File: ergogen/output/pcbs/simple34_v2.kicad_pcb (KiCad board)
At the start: 2 copper layers, 122.2 x 90.8 mm, 42 parts

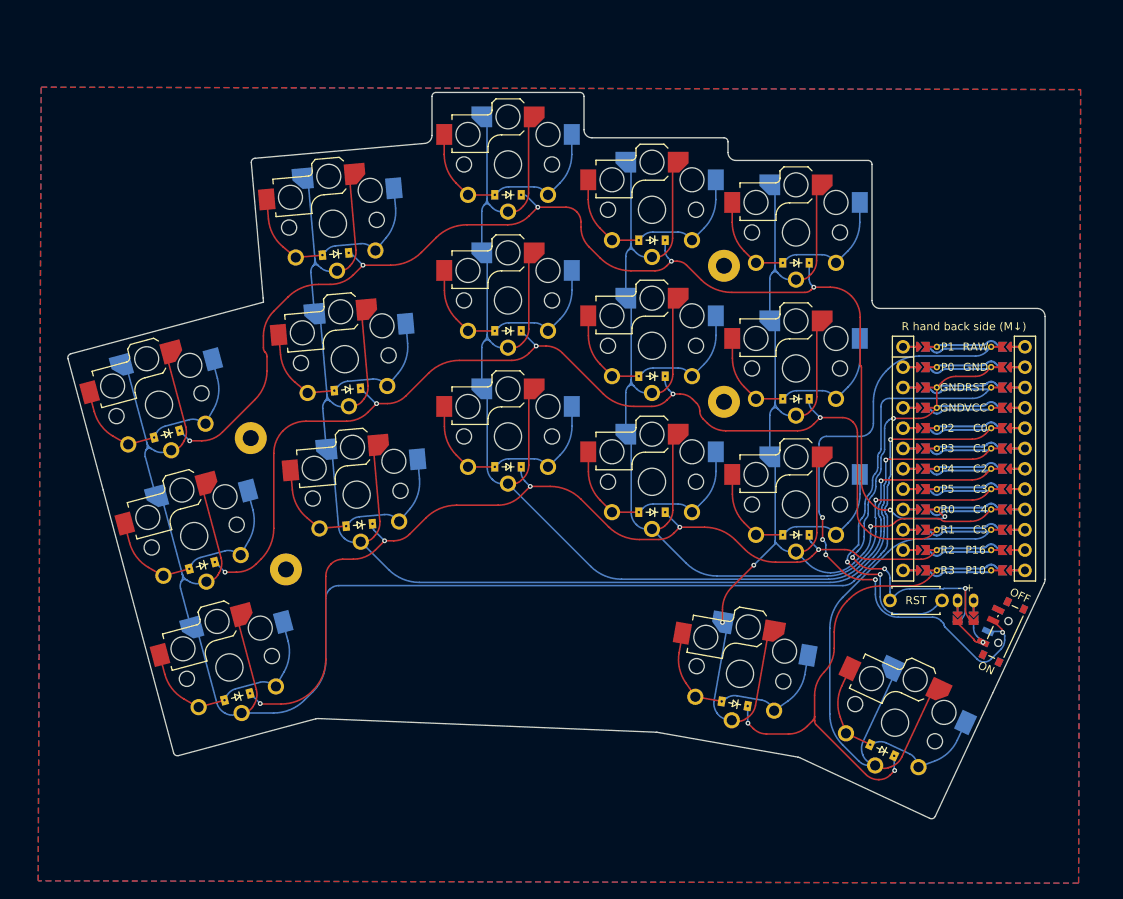
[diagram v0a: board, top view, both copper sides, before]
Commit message: OH MY, ARCS EXISTS
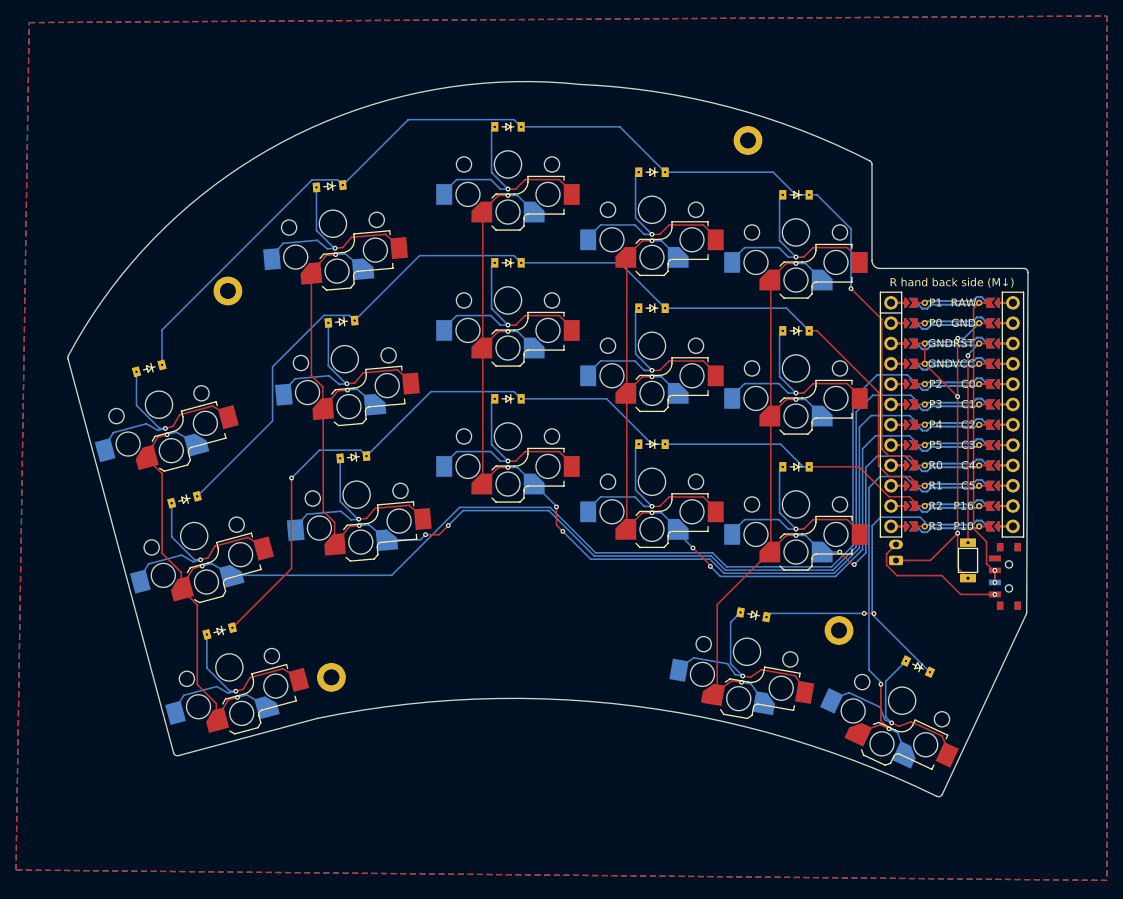
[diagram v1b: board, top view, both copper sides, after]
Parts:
- removed RST1: , ceoloide:reset_switch_tht_top
- added SW1: , local:reset_smd, F.Cu at (137.9, 87.2)
- moved H4 32.0 mm to (121.8, 96.0), turned to -17.5 degrees
- moved H1 18.6 mm to (45.4, 53.5)
- moved H2 16.0 mm to (110.4, 34.7)
- moved H3 14.6 mm to (58.4, 101.8)
- moved D17 11.4 mm to (131.7, 100.5)
- moved D16 11.4 mm to (111.1, 94.0)
- moved JST1 10.6 mm to (128.9, 86.2), turned to 90 degrees
- moved D6 8.50 mm to (58.1, 40.4)
- moved D4 8.50 mm to (61.1, 74.3)
- moved D5 8.50 mm to (59.6, 57.4)
- moved D14 8.50 mm to (116.4, 58.5)
- moved D10 8.50 mm to (98.4, 72.7)
- moved D12 8.50 mm to (98.4, 38.7)
- moved D13 8.50 mm to (116.4, 75.5)
- moved D15 8.50 mm to (116.4, 41.5)
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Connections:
- JST1 pad 1: BAT_P -> GND
- JST1 pad 2: GND -> BAT_P
- S1 pad 1: pinky_bottom -> C0
- S10 pad 1: index_bottom -> C3
- S11 pad 1: index_home -> C3
- S12 pad 1: index_top -> C3
- S13 pad 1: inner_bottom -> C4
- S14 pad 1: inner_home -> C4
- S15 pad 1: inner_top -> C4
- S16 pad 1: first_only -> C4
- S17 pad 1: second_only -> C5
- S2 pad 1: pinky_home -> C0
- S3 pad 1: pinky_top -> C0
- S4 pad 1: ring_bottom -> C1
- S5 pad 1: ring_home -> C1
- S6 pad 1: ring_top -> C1
- S7 pad 1: middle_bottom -> C2
- S8 pad 1: middle_home -> C2
- S9 pad 1: middle_top -> C2
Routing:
- net C4: track 177.6 -> 122.3 mm, vias 3 -> 6
- net C0: track 229.2 -> 184.3 mm, vias 1 -> 3
- net C3: track 159.5 -> 116.6 mm, vias 1 -> 5
- net C2: track 182.7 -> 140.1 mm, vias 1 -> 5
- net C1: track 200.9 -> 160.0 mm, vias 1 -> 5
- net RAW: track 88.5 -> 47.8 mm, vias 5 -> 2
- net C5: track 83.2 -> 56.0 mm, vias 0 -> 2
- net RST: track 62.1 -> 35.3 mm, vias 2 -> 1
- net R1: track 148.4 -> 134.1 mm, vias 5 -> 0
- net R0: track 165.5 -> 151.7 mm, vias 7 -> 1
- net R3: track 65.5 -> 52.6 mm
- net BAT_P: track 7.03 -> 18.1 mm
- net GND: track 91.0 -> 81.0 mm, vias 4 -> 3
- net R2: track 129.5 -> 120.8 mm, vias 5 -> 1
- net JST1_2: track 3.60 -> 0.00 mm
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- added copper zone on B.Cu, net GND
- added copper zone on F.Cu, net GND
- removed copper zone on B.Cu, net (none)
- removed copper zone on F.Cu, net (none)
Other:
- board size 122.2 x 90.8 mm -> 120 x 89.4 mm
- board text removed: "- +"

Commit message: case fillet
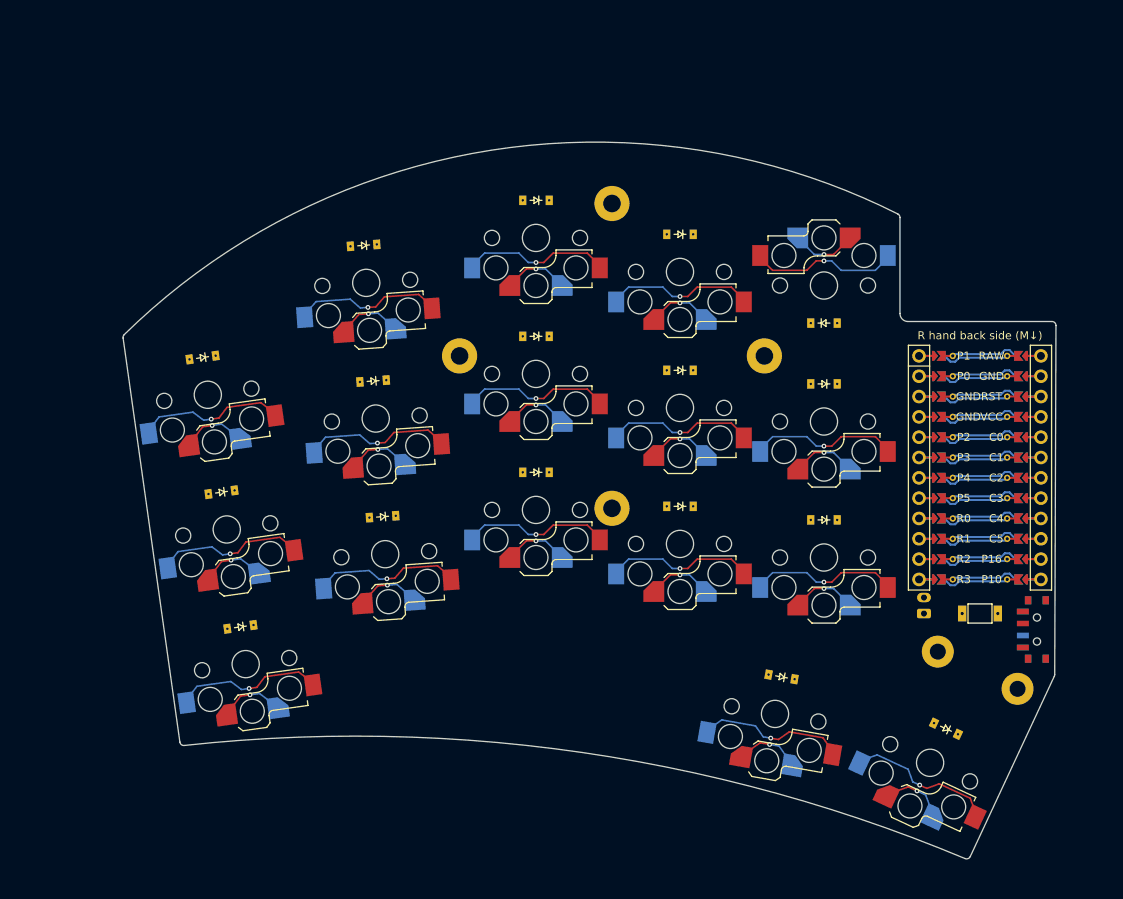
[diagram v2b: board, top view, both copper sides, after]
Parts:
- removed H3, H4: , ceoloide:mounting_hole_plated
- added TP1: Tenting Puck, no hole, TentingPuck_NoHole, B.Cu at (93.4, 61.6)
- moved H1 99.5 mm to (134.2, 98.6), turned to -25 degrees
- moved H2 76.4 mm to (144.1, 103.3), turned to -25 degrees
- moved D15 16.4 mm to (119.9, 57.5), turned to 360 degrees
- moved S7 9.83 mm to (83.9, 80.9)
- moved D8 9.83 mm to (83.9, 59.2)
- moved D9 9.83 mm to (83.9, 42.2)
- moved S8 9.83 mm to (83.9, 63.9)
- moved S9 9.83 mm to (83.9, 46.9)
- moved D7 9.83 mm to (83.9, 76.2)
- moved D6 8.52 mm to (62.4, 47.8), turned to 184 degrees
- moved D10 8.52 mm to (101.9, 80.4)
- moved S11 8.52 mm to (101.9, 68.1)
- moved S12 8.52 mm to (101.9, 51.1)
- moved D11 8.52 mm to (101.9, 63.4)
- moved D12 8.52 mm to (101.9, 46.4)
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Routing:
- net (no net): track 0.00 -> 337.7 mm
- net C0: track 184.3 -> 24.8 mm
- net R0: track 151.7 -> 0.00 mm, vias 1 -> 0
- net C1: track 160.0 -> 24.8 mm, vias 5 -> 3
- net R1: track 134.1 -> 0.00 mm
- net R2: track 120.8 -> 0.00 mm, vias 1 -> 0
- net C2: track 140.1 -> 24.8 mm, vias 5 -> 3
- net C3: track 116.6 -> 24.8 mm, vias 5 -> 3
- net C4: track 122.3 -> 33.1 mm, vias 6 -> 4
- net GND: track 81.0 -> 0.00 mm, vias 3 -> 0
- net R3: track 52.6 -> 0.00 mm, vias 2 -> 0
- net RAW: track 47.8 -> 0.00 mm, vias 2 -> 0
- net C5: track 56.0 -> 8.27 mm, vias 2 -> 1
- net RST: track 35.3 -> 0.00 mm, vias 1 -> 0
- net BAT_P: track 18.1 -> 0.00 mm, vias 1 -> 0
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- removed copper zone on B.Cu, net GND
- removed copper zone on F.Cu, net GND
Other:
- board size 120 x 89.4 mm -> 116.6 x 89.6 mm
